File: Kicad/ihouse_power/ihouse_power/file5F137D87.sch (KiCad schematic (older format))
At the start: 35 parts, among them J12 OPTIC, J14 OPT1, J15 LEAK1, J16 LEAK2, J17 LEAK3, J18 DHT22, J23 Valve1, J24 Valve2, J25 Conn_01x14, J26 Valve1, J27 Valve2, J28 OPT2, J29 OPT3, U6 LM393, U7 LM393

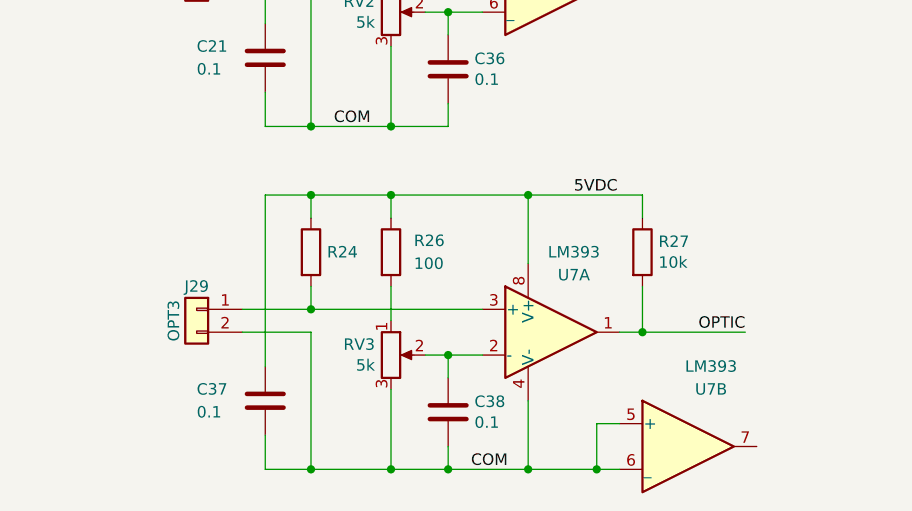
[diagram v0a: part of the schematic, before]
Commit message: schemos korekcijos ir ploksciu paruosimas
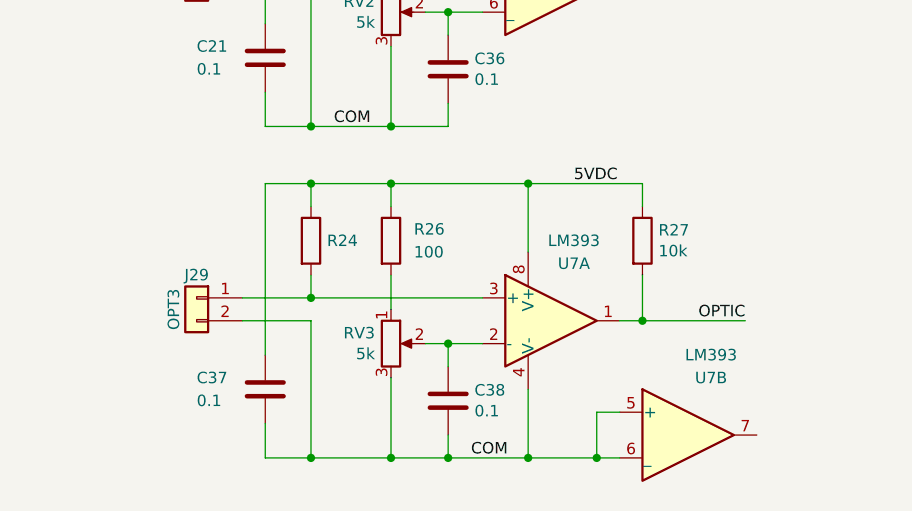
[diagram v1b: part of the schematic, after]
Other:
- moved on the sheet: C37, C38, J29, R24, R26, R27, RV3, U7A, U7B
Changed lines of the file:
@@
 L Device:R R24
 U 1 1 5D1CD8A1
-P 5750 4300
-F 0 "R24" H 5820 4300 50  0000 L CNN
-F 1 "R" H 5820 4255 50  0001 L CNN
-F 2 "Resistor_SMD:R_0805_2012Metric_Pad1.15x1.40mm_HandSolder" V 5680 4300 50  0001 C CNN
-F 3 "~" H 5750 4300 50  0001 C CNN
-	1    5750 4300
+P 5750 4250
+F 0 "R24" H 5820 4250 50  0000 L CNN
+F 1 "R" H 5820 4205 50  0001 L CNN
+F 2 "Resistor_SMD:R_0805_2012Metric_Pad1.15x1.40mm_HandSolder" V 5680 4250 50  0001 C CNN
+F 3 "~" H 5750 4250 50  0001 C CNN
+	1    5750 4250
 	1    0    0    -1
 $EndComp
 Wire Wire Line
-	5750 4450 5750 4550
+	5750 4400 5750 4500
 Wire Wire Line
-	5750 4550 5450 4550
+	5750 4500 5450 4500
 Wire Wire Line
-	6700 4950 6700 5250
-Text Label 6450 5250 0    50   ~ 0
+	6700 4900 6700 5200
+Text Label 6450 5200 0    50   ~ 0
 COM
 Wire Wire Line
-	5750 4550 6500 4550
-Connection ~ 5750 4550
+	5750 4500 6500 4500
+Connection ~ 5750 4500
 Wire Wire Line
-	5750 4150 5750 4050
+	5750 4100 5750 4000
 Wire Wire Line
-	6700 4050 6700 4350
+	6700 4000 6700 4300
 Wire Wire Line
-	7200 4650 7100 4650
+	7200 4600 7100 4600
 $Comp
 L Device:R R27
 U 1 1 5D1CD8B0
-P 7200 4300
-F 0 "R27" H 7270 4346 50  0000 L CNN
-F 1 "10k" H 7270 4255 50  0000 L CNN
-F 2 "Resistor_SMD:R_0805_2012Metric_Pad1.15x1.40mm_HandSolder" V 7130 4300 50  0001 C CNN
-F 3 "~" H 7200 4300 50  0001 C CNN
-	1    7200 4300
+P 7200 4250
+F 0 "R27" H 7270 4296 50  0000 L CNN
+F 1 "10k" H 7270 4205 50  0000 L CNN
+F 2 "Resistor_SMD:R_0805_2012Metric_Pad1.15x1.40mm_HandSolder" V 7130 4250 50  0001 C CNN
+F 3 "~" H 7200 4250 50  0001 C CNN
+	1    7200 4250
 	1    0    0    -1
 $EndComp
 Wire Wire Line
-	7200 4450 7200 4650
-Connection ~ 7200 4650
+	7200 4400 7200 4600
+Connection ~ 7200 4600
 Wire Wire Line
-	6700 4050 7200 4050
+	6700 4000 7200 4000
 Wire Wire Line
-	7200 4050 7200 4150
-Connection ~ 6700 4050
+	7200 4000 7200 4100
+Connection ~ 6700 4000
 $Comp
 L Comparator:LM393 U7
 U 1 1 5D1CD8BB
-P 6800 4650
-F 0 "U7" H 6900 4900 50  0000 C CNN
-F 1 "LM393" H 6900 5000 50  0000 C CNN
-F 2 "Package_SO:SOIC-8_3.9x4.9mm_P1.27mm" H 6800 4650 50  0001 C CNN
-F 3 "http://www.ti.com/lit/ds/symlink/lm393-n.pdf" H 6800 4650 50  0001 C CNN
-	1    6800 4650
+P 6800 4600
+F 0 "U7" H 6900 4850 50  0000 C CNN
+F 1 "LM393" H 6900 4950 50  0000 C CNN
+F 2 "Package_SO:SOIC-8_3.9x4.9mm_P1.27mm" H 6800 4600 50  0001 C CNN
+F 3 "http://www.ti.com/lit/ds/symlink/lm393-n.pdf" H 6800 4600 50  0001 C CNN
+	1    6800 4600
 	1    0    0    -1
 $EndComp
@@
 L Comparator:LM393 U7
 U 3 1 5D1CD8C1
-P 6800 4650
-F 0 "U7" H 6758 4696 50  0001 L CNN
-F 1 "LM393" H 6758 4605 50  0001 L CNN
-F 2 "" H 6800 4650 50  0001 C CNN
-F 3 "http://www.ti.com/lit/ds/symlink/lm393-n.pdf" H 6800 4650 50  0001 C CNN
-	3    6800 4650
+P 6800 4600
+F 0 "U7" H 6758 4646 50  0001 L CNN
+F 1 "LM393" H 6758 4555 50  0001 L CNN
+F 2 "" H 6800 4600 50  0001 C CNN
+F 3 "http://www.ti.com/lit/ds/symlink/lm393-n.pdf" H 6800 4600 50  0001 C CNN
+	3    6800 4600
 	1    0    0    -1
 $EndComp
-Text Label 6900 4050 0    50   ~ 0
+Text Label 6900 4000 0    50   ~ 0
 5VDC
 $Comp
 L Connector_Generic:Conn_01x02 J29
 U 1 1 5D1CD8CA
-P 5250 4550
-F 0 "J29" H 5250 4650 50  0000 C CNN
-F 1 "OPT3" V 5350 4500 50  0000 C CNN
-F 2 "Connector_JST:JST_EH_B2B-EH-A_1x02_P2.50mm_Vertical" H 5250 4550 50  0001 C CNN
-F 3 "~" H 5250 4550 50  0001 C CNN
-	1    5250 4550
+P 5250 4500
+F 0 "J29" H 5250 4600 50  0000 C CNN
+F 1 "OPT3" V 5350 4450 50  0000 C CNN
+F 2 "Connector_JST:JST_EH_B2B-EH-A_1x02_P2.50mm_Vertical" H 5250 4500 50  0001 C CNN
+F 3 "~" H 5250 4500 50  0001 C CNN
+	1    5250 4500
 	-1   0    0    -1
 $EndComp
 Wire Wire Line
-	5450 4650 5750 4650
+	5450 4600 5750 4600
 Wire Wire Line
-	5750 5250 6100 5250
+	5750 5200 6100 5200
 $Comp
 L Device:R_POT RV3
 U 1 1 5D1CD8D3
-P 6100 4750
-F 0 "RV3" H 6030 4796 50  0000 R CNN
-F 1 "5k" H 6030 4705 50  0000 R CNN
-F 2 "Potentiometer_THT:Potentiometer_Piher_PT-6-V_Vertical" H 6100 4750 50  0001 C CNN
-F 3 "~" H 6100 4750 50  0001 C CNN
-	1    6100 4750
+P 6100 4700
+F 0 "RV3" H 6030 4746 50  0000 R CNN
+F 1 "5k" H 6030 4655 50  0000 R CNN
+F 2 "Potentiometer_THT:Potentiometer_Piher_PT-6-V_Vertical" H 6100 4700 50  0001 C CNN
+F 3 "~" H 6100 4700 50  0001 C CNN
+	1    6100 4700
 	1    0    0    -1
 $EndComp
 Wire Wire Line
-	5750 4050 6100 4050
+	5750 4000 6100 4000
 Wire Wire Line
-	5750 4650 5750 5250
+	5750 4600 5750 5200
 Wire Wire Line
-	6250 4750 6350 4750
+	6250 4700 6350 4700
 Wire Wire Line
-	6100 4900 6100 5250
-Connection ~ 6100 5250
+	6100 4850 6100 5200
+Connection ~ 6100 5200
 Wire Wire Line
-	6100 5250 6350 5250
+	6100 5200 6350 5200
 Wire Wire Line
-	6100 4600 6100 4450
-Connection ~ 6100 4050
+	6100 4550 6100 4400
+Connection ~ 6100 4000
 Wire Wire Line
-	6100 4050 6700 4050
+	6100 4000 6700 4000
 $Comp
 L Device:C C38
 U 1 1 5D1CD8E2
-P 6350 5000
-F 0 "C38" H 6465 5046 50  0000 L CNN
-F 1 "0.1" H 6465 4955 50  0000 L CNN
-F 2 "Capacitor_SMD:C_0805_2012Metric" H 6388 4850 50  0001 C CNN
-F 3 "~" H 6350 5000 50  0001 C CNN
-	1    6350 5000
+P 6350 4950
+F 0 "C38" H 6465 4996 50  0000 L CNN
+F 1 "0.1" H 6465 4905 50  0000 L CNN
+F 2 "Capacitor_SMD:C_0805_2012Metric" H 6388 4800 50  0001 C CNN
+F 3 "~" H 6350 4950 50  0001 C CNN
+	1    6350 4950
 	1    0    0    -1
 $EndComp
 Wire Wire Line
-	6350 4850 6350 4750
-Connection ~ 6350 4750
+	6350 4800 6350 4700
+Connection ~ 6350 4700
 Wire Wire Line
-	6350 4750 6500 4750
+	6350 4700 6500 4700
 Wire Wire Line
-	6350 5150 6350 5250
-Connection ~ 6350 5250
+	6350 5100 6350 5200
+Connection ~ 6350 5200
 Wire Wire Line
-	6350 5250 6700 5250
+	6350 5200 6700 5200
 $Comp
 L Device:R R26
 U 1 1 5D1CD8F1
-P 6100 4300
-F 0 "R26" H 6200 4350 50  0000 L CNN
-F 1 "100" H 6200 4250 50  0000 L CNN
-F 2 "Resistor_SMD:R_0805_2012Metric_Pad1.15x1.40mm_HandSolder" V 6030 4300 50  0001 C CNN
-F 3 "~" H 6100 4300 50  0001 C CNN
-	1    6100 4300
+P 6100 4250
+F 0 "R26" H 6200 4300 50  0000 L CNN
+F 1 "100" H 6200 4200 50  0000 L CNN
+F 2 "Resistor_SMD:R_0805_2012Metric_Pad1.15x1.40mm_HandSolder" V 6030 4250 50  0001 C CNN
+F 3 "~" H 6100 4250 50  0001 C CNN
+	1    6100 4250
 	1    0    0    -1
 $EndComp
 Wire Wire Line
-	6100 4150 6100 4050
+	6100 4100 6100 4000
 $Comp
 L Device:C C37
 U 1 1 5D1D276C
-P 5550 4950
-F 0 "C37" H 5250 5000 50  0000 L CNN
-F 1 "0.1" H 5250 4900 50  0000 L CNN
-F 2 "Capacitor_SMD:C_0805_2012Metric" H 5588 4800 50  0001 C CNN
-F 3 "~" H 5550 4950 50  0001 C CNN
-	1    5550 4950
+P 5550 4900
+F 0 "C37" H 5250 4950 50  0000 L CNN
+F 1 "0.1" H 5250 4850 50  0000 L CNN
+F 2 "Capacitor_SMD:C_0805_2012Metric" H 5588 4750 50  0001 C CNN
+F 3 "~" H 5550 4900 50  0001 C CNN
+	1    5550 4900
 	1    0    0    -1
 $EndComp
 Wire Wire Line
-	5750 4050 5550 4050
+	5750 4000 5550 4000
 Wire Wire Line
-	5550 4050 5550 4800
-Connection ~ 5750 4050
+	5550 4000 5550 4750
+Connection ~ 5750 4000
 Wire Wire Line
-	5550 5100 5550 5250
+	5550 5050 5550 5200
 Wire Wire Line
-	5550 5250 5750 5250
-Connection ~ 5750 5250
+	5550 5200 5750 5200
+Connection ~ 5750 5200
 Text Label 2400 1600 0    50   ~ 0
 OPTIC
-Text Label 7650 4650 2    50   ~ 0
+Text Label 7650 4600 2    50   ~ 0
 OPTIC
 Wire Wire Line
-	7200 4650 7650 4650
+	7200 4600 7650 4600
 $Comp
 L Comparator:LM393 U7
 U 2 1 5D229F22
-P 7400 5150
-F 0 "U7" H 7500 5400 50  0000 C CNN
-F 1 "LM393" H 7500 5500 50  0000 C CNN
-F 2 "Package_SO:SOIC-8_3.9x4.9mm_P1.27mm" H 7400 5150 50  0001 C CNN
-F 3 "http://www.ti.com/lit/ds/symlink/lm393-n.pdf" H 7400 5150 50  0001 C CNN
-	2    7400 5150
+P 7400 5100
+F 0 "U7" H 7500 5350 50  0000 C CNN
+F 1 "LM393" H 7500 5450 50  0000 C CNN
+F 2 "Package_SO:SOIC-8_3.9x4.9mm_P1.27mm" H 7400 5100 50  0001 C CNN
+F 3 "http://www.ti.com/lit/ds/symlink/lm393-n.pdf" H 7400 5100 50  0001 C CNN
+	2    7400 5100
 	1    0    0    -1
 $EndComp
 Wire Wire Line
-	7100 5050 7000 5050
+	7100 5000 7000 5000
 Wire Wire Line
-	7000 5050 7000 5250
+	7000 5000 7000 5200
 Wire Wire Line
-	7000 5250 7100 5250
+	7000 5200 7100 5200
 Wire Wire Line
-	7000 5250 6700 5250
-Connection ~ 7000 5250
-Connection ~ 6700 5250
+	7000 5200 6700 5200
+Connection ~ 7000 5200
+Connection ~ 6700 5200
 Text Label 1550 3200 0    50   ~ 0
 DATA
